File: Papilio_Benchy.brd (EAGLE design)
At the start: 101.6 x 55.9 mm, 122 parts, among them IC1 FT2232H, SW1 SWITCH-2CH-6P-3010010P1, SW2 EVQQ2, T100 MOSFET-NCHANNELSMD, U1 ARDUINO_MEGA_SHIELD, U100 PCA9306, U101 ATMEGA32U4-XUMU, U2 LTC3419EMS, U3 93C46B, X1 12MHz, Y1 16MHz KX-7

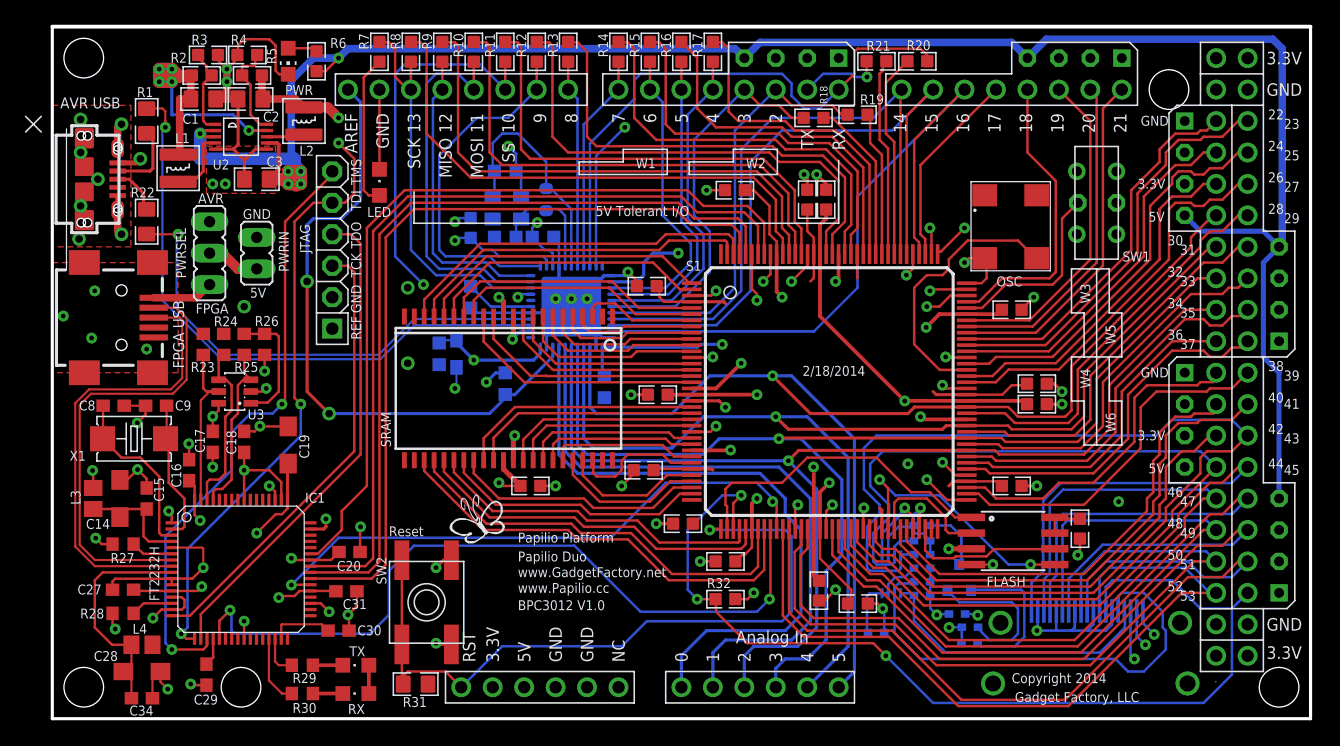
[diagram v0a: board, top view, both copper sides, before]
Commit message: Final fixes as pointed out in the forum.
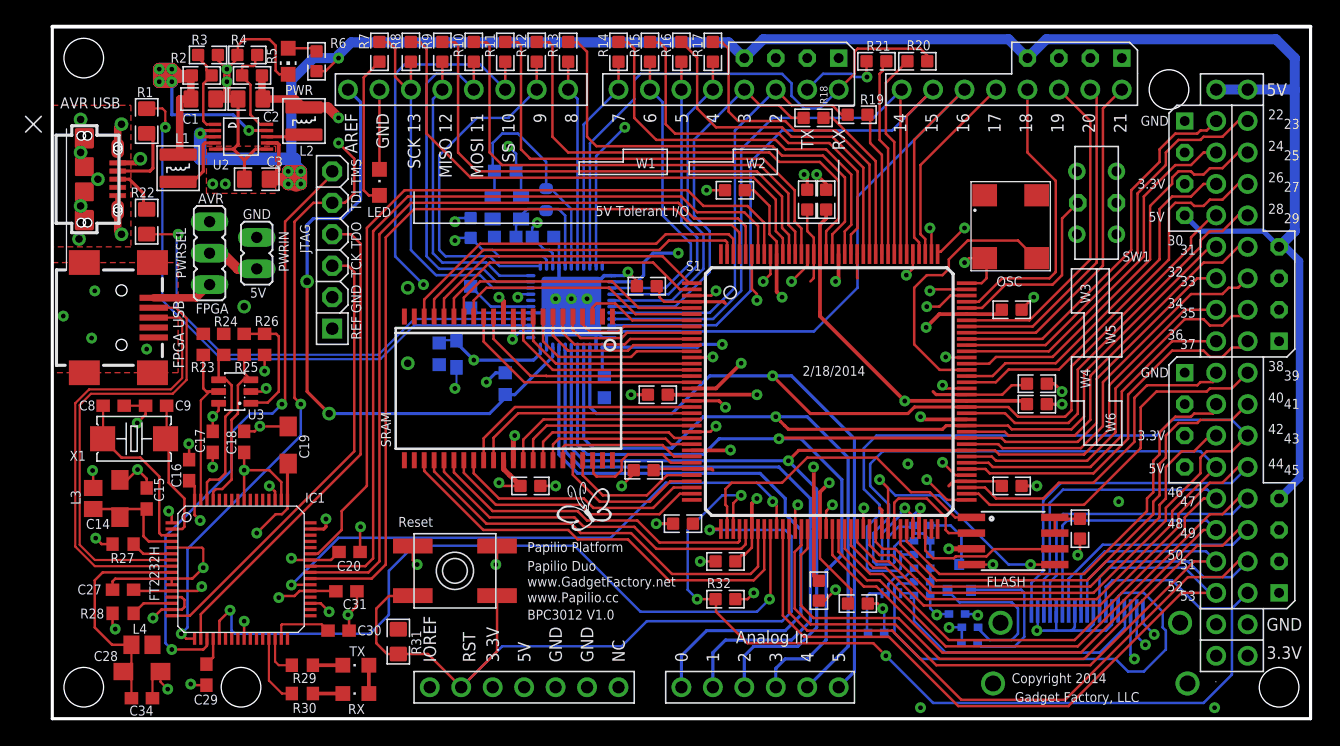
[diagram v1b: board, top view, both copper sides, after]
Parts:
- moved U$7 8.70 mm to (40.5, 14.6)
- moved R31 3.70 mm to (27.9, 6.22), turned to 90 degrees
- moved SW2 3.42 mm to (32.5, 11.9), turned to 0 degrees
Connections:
- net 3V3: now also U1.IOREF; no longer U1.3V3@3, U1.3V3@4
- net 5V0: now also U1.5V@1, U1.5V@2
- net GND: no longer U1.GND@5, U1.GND@6
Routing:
- net 5V0: track 297.1 -> 305.8 mm
- net RESET: track 59.1 -> 66.1 mm
- net GND: track 228.4 -> 229.3 mm
- net 1V2: track 149.6 -> 149.0 mm
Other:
- board text added: "Bottom silkscreen is on layer 200"
- board text added: "Top silkscreen is on layer 130: tSilk"
